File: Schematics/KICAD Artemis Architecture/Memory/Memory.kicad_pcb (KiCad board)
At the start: 4 copper layers, 100.1 x 45.8 mm, 11 parts, among them IC1 AT28C64B-15PU, IC2 AS7C164A-15PCN, IC3 AT28C64B-15PU, IC4 AS7C164A-15PCN, J1 Bus LB, J2 Bus UB, J3 Control, J4 Power, J5 Address, U1 74LS00

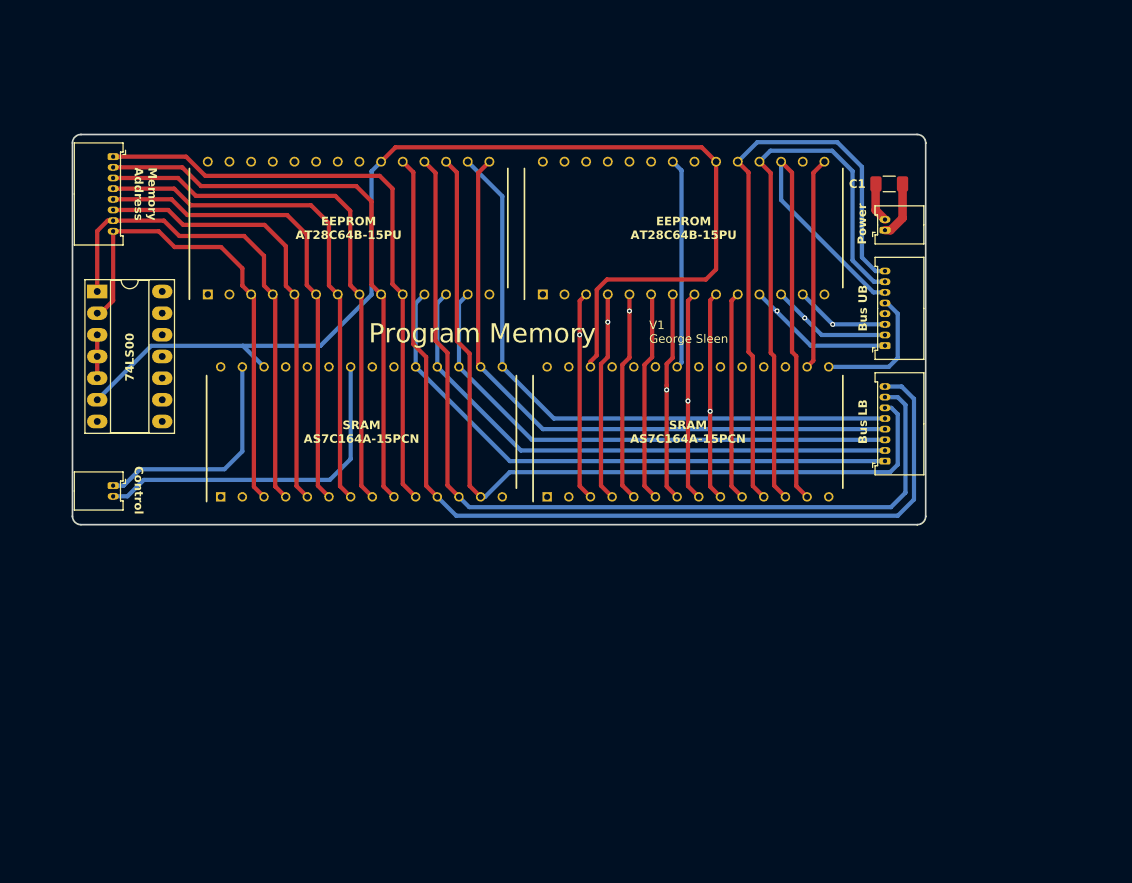
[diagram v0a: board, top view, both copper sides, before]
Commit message: Memory rework pt.1
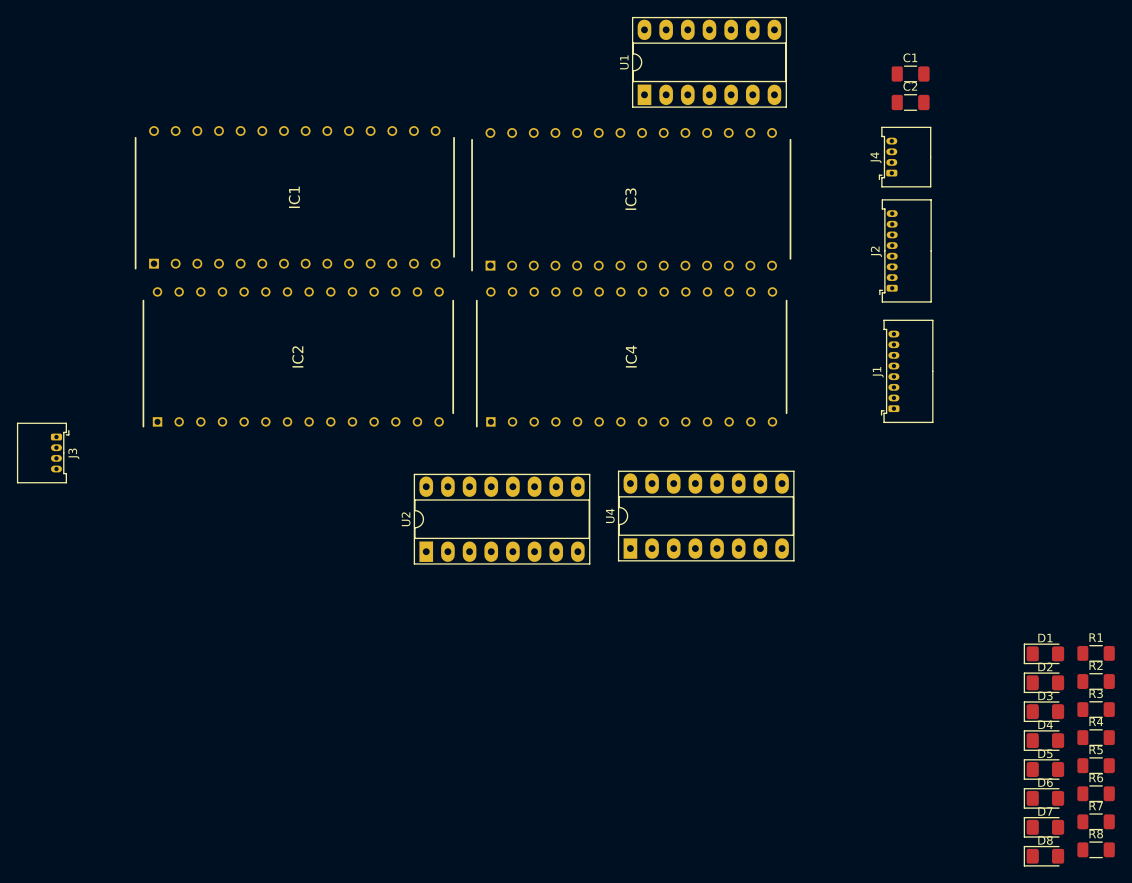
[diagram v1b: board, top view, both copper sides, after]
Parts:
- removed J5: Address, Connector_Molex:Molex_PicoBlade_53048-0810_1x08_P1.25mm_Horizontal
- added C2: 0.1 uF, Capacitor_SMD:C_1206_3216Metric_Pad1.33x1.80mm_HandSolder, F.Cu at (195.5, 50.2)
- added D1: LED, LED_SMD:LED_1206_3216Metric_Pad1.42x1.75mm_HandSolder, F.Cu at (211.3, 114.9)
- added D2: LED, LED_SMD:LED_1206_3216Metric_Pad1.42x1.75mm_HandSolder, F.Cu at (211.3, 118.3)
- added D3: LED, LED_SMD:LED_1206_3216Metric_Pad1.42x1.75mm_HandSolder, F.Cu at (211.3, 121.7)
- added D4: LED, LED_SMD:LED_1206_3216Metric_Pad1.42x1.75mm_HandSolder, F.Cu at (211.3, 125.1)
- added D5: LED, LED_SMD:LED_1206_3216Metric_Pad1.42x1.75mm_HandSolder, F.Cu at (211.3, 128.5)
- added D6: LED, LED_SMD:LED_1206_3216Metric_Pad1.42x1.75mm_HandSolder, F.Cu at (211.3, 131.8)
- added D7: LED, LED_SMD:LED_1206_3216Metric_Pad1.42x1.75mm_HandSolder, F.Cu at (211.3, 135.2)
- added D8: LED, LED_SMD:LED_1206_3216Metric_Pad1.42x1.75mm_HandSolder, F.Cu at (211.3, 138.6)
- added R1: 220, Resistor_SMD:R_1206_3216Metric_Pad1.30x1.75mm_HandSolder, F.Cu at (217.2, 114.8)
- added R2: 220, Resistor_SMD:R_1206_3216Metric_Pad1.30x1.75mm_HandSolder, F.Cu at (217.2, 118.1)
- added R3: 220, Resistor_SMD:R_1206_3216Metric_Pad1.30x1.75mm_HandSolder, F.Cu at (217.2, 121.4)
- added R4: 220, Resistor_SMD:R_1206_3216Metric_Pad1.30x1.75mm_HandSolder, F.Cu at (217.2, 124.7)
- added R5: 220, Resistor_SMD:R_1206_3216Metric_Pad1.30x1.75mm_HandSolder, F.Cu at (217.2, 128.0)
- added R6: 220, Resistor_SMD:R_1206_3216Metric_Pad1.30x1.75mm_HandSolder, F.Cu at (217.2, 131.3)
- added R7: 220, Resistor_SMD:R_1206_3216Metric_Pad1.30x1.75mm_HandSolder, F.Cu at (217.2, 134.6)
- added R8: 220, Resistor_SMD:R_1206_3216Metric_Pad1.30x1.75mm_HandSolder, F.Cu at (217.2, 137.9)
- added U2: 74LS173, Package_DIP:DIP-16_W7.62mm_Socket_LongPads, F.Cu at (138.7, 102.9)
- added U4: 74LS173, Package_DIP:DIP-16_W7.62mm_Socket_LongPads, F.Cu at (162.7, 102.5)
- J3, J4: footprint Connector_Molex:Molex_PicoBlade_53048-0210_1x02_P1.25mm_Horizontal -> Connector_Molex:Molex_PicoBlade_53048-0410_1x04_P1.25mm_Horizontal
- moved U1 68.2 mm to (164.3, 49.4), turned to 90 degrees
- moved C1 13.1 mm to (195.5, 46.9), turned to 0 degrees
- moved IC2 11.5 mm to (123.7, 80.1)
- moved IC4 11.0 mm to (162.8, 80.1)
- moved J3 8.76 mm to (95.3, 89.5)
- moved IC1 7.26 mm to (123.3, 61.4)
- moved IC3 7.00 mm to (162.8, 61.6)
- moved J2 6.79 mm to (193.3, 72.0)
- moved J4 6.75 mm to (193.3, 58.5)
- moved J1 6.24 mm to (193.6, 86.2)
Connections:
- net /A0 renamed Net-(D8-A)
- net /A1 renamed Net-(D7-A)
- net /A2 renamed Net-(D6-A)
- net /A3 renamed Net-(D5-A)
- net /A4 renamed Net-(D4-A)
- net /A5 renamed Net-(D3-A)
- net /A6 renamed Net-(D2-A)
- net /A7 renamed Net-(D1-A)
- IC1 pad 22: /~{MR} -> /~{MvR}
- IC2 pad 22: /~{MR} -> /~{MvR}
- IC2 pad 27: /~{MW} -> /~{MvW}
- IC3 pad 22: /~{MR} -> /~{MvR}
- IC4 pad 22: /~{MR} -> /~{MvR}
- IC4 pad 27: /~{MW} -> /~{MvW}
- J3 pad 1: /~{MW} -> /~{MaI}
- J3 pad 2: /~{MR} -> /~{MvW}
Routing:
- net /~{MR}: track 146.0 -> 0.00 mm
- net Net-(D8-A): track 135.7 -> 0.00 mm
- net Net-(IC1-~{CE}): track 134.5 -> 0.00 mm
- net Net-(D7-A): track 133.4 -> 0.00 mm, vias 1 -> 0
- net Net-(D6-A): track 130.3 -> 0.00 mm, vias 1 -> 0
- net Net-(D5-A): track 126.9 -> 0.00 mm, vias 1 -> 0
- net Net-(D2-A): track 123.4 -> 0.00 mm, vias 1 -> 0
- net Net-(D4-A): track 121.8 -> 0.00 mm
- net Net-(D1-A): track 120.5 -> 0.00 mm, vias 1 -> 0
- net Net-(D3-A): track 117.2 -> 0.00 mm, vias 1 -> 0
- net /BUS 7: track 114.4 -> 0.00 mm
- net /BUS 6: track 107.6 -> 0.00 mm
- net /BUS 5: track 99.2 -> 0.00 mm
- net /BUS 3: track 75.2 -> 0.00 mm
- net /BUS 4: track 73.1 -> 0.00 mm
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- removed copper zone on In1.Cu, net GNDREF
- removed copper zone on In2.Cu, net VCC
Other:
- board outline removed
- board text removed: "74LS00"
- board text removed: "Bus LB"
- board text removed: "Bus UB"
- board text removed: "Control"
- board text removed: "EEPROM AT28C64B-15PU"
- board text removed: "Memory Address"
- board text removed: "Power"
- board text removed: "Program Memory"
- board text removed: "SRAM AS7C164A-15PCN"
- board text removed: "V1 George Sleen"

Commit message: Program Memory PCB
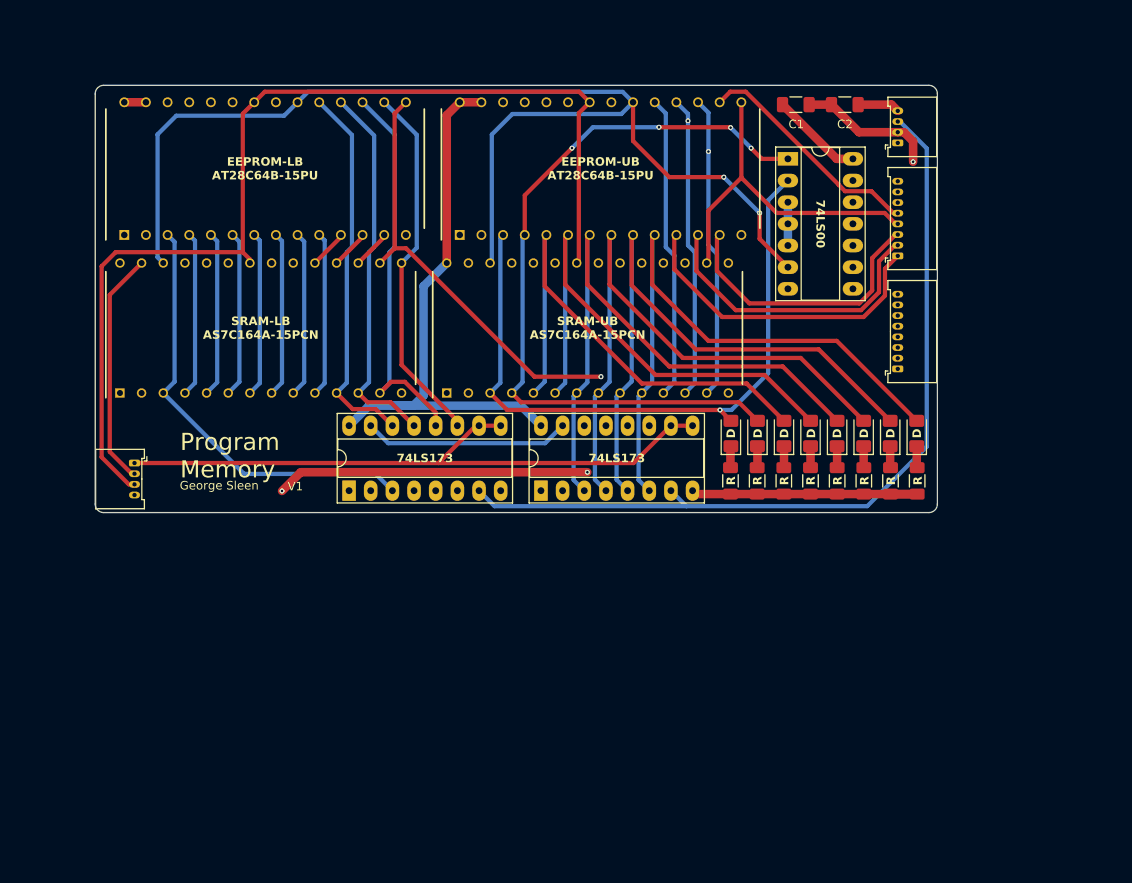
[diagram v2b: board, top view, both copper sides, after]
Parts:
- moved D8 51.8 mm to (196.2, 89.1), turned to 90 degrees
- moved D7 49.6 mm to (193.1, 89.1), turned to 90 degrees
- moved R8 48.1 mm to (196.3, 94.6), turned to -90 degrees
- moved D6 47.8 mm to (190.0, 89.1), turned to 90 degrees
- moved R1 47.4 mm to (174.4, 94.6), turned to -90 degrees
- moved R7 46.7 mm to (193.1, 94.6), turned to -90 degrees
- moved D5 46.3 mm to (186.9, 89.1), turned to 90 degrees
- moved R2 46.2 mm to (177.5, 94.6), turned to -90 degrees
- moved R6 45.7 mm to (190.0, 94.6), turned to -90 degrees
- moved R3 45.4 mm to (180.6, 94.6), turned to -90 degrees
- moved D4 45.3 mm to (183.8, 89.1), turned to 90 degrees
- moved R5 45.1 mm to (186.9, 94.6), turned to -90 degrees
- moved R4 45.0 mm to (183.8, 94.6), turned to -90 degrees
- moved D 45.0 mm to (174.4, 89.1), turned to 90 degrees
- moved D3 44.8 mm to (180.7, 89.1), turned to 90 degrees
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- renumbered D1 to D
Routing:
- net Net-(IC1-~{CE}): track 0.00 -> 177.2 mm, vias 0 -> 2
- net VCC: track 0.00 -> 175.9 mm, vias 0 -> 2
- net Net-(D2-A): track 0.00 -> 161.1 mm, vias 0 -> 4
- net Net-(D1-A): track 0.00 -> 149.7 mm, vias 0 -> 1
- net Net-(D5-A): track 0.00 -> 136.4 mm
- net Net-(D8-A): track 0.00 -> 135.3 mm
- net Net-(D7-A): track 0.00 -> 134.7 mm
- net Net-(D6-A): track 0.00 -> 133.3 mm
- net Net-(D4-A): track 0.00 -> 130.6 mm
- net Net-(D3-A): track 0.00 -> 130.5 mm
- net /~{MvR}: track 0.00 -> 124.4 mm
- net /BUS 7: track 0.00 -> 114.5 mm
- net /BUS 2: track 0.00 -> 112.9 mm
- net /BUS 1: track 0.00 -> 112.8 mm
- net /BUS 0: track 0.00 -> 112.8 mm
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- added copper zone on In1.Cu, net GNDREF
- added copper zone on In2.Cu, net VCC
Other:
- board outline added: 98.8 x 50.1 mm
- board text added: "74LS00"
- board text added: "74LS173"
- board text added: "D"
- board text added: "EEPROM-LB AT28C64B-15PU"
- board text added: "EEPROM-UB AT28C64B-15PU"
- board text added: "George Sleen"
- board text added: "Program Memory"
- board text added: "R"
- board text added: "SRAM-LB AS7C164A-15PCN"
- board text added: "SRAM-UB AS7C164A-15PCN"
- board text added: "V1"
